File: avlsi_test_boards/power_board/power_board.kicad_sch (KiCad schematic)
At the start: 2 parts, among them J1 PJ-102AH, J2 PJ-102AH

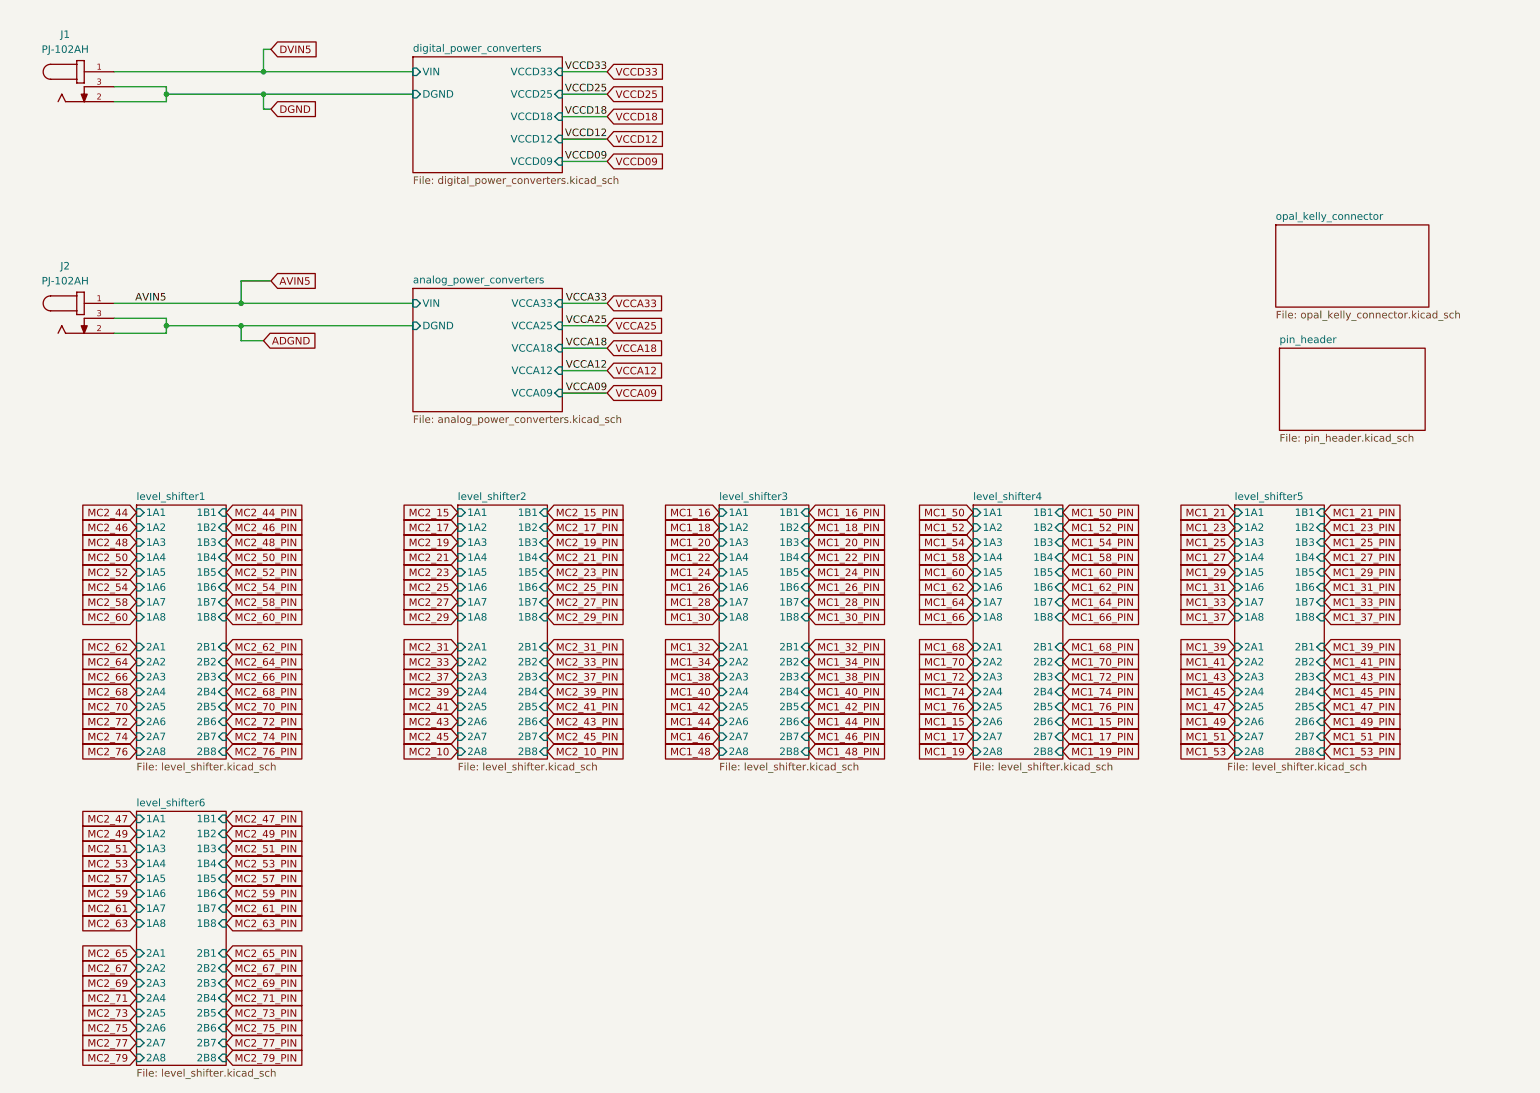
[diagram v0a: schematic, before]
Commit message: Update schematic
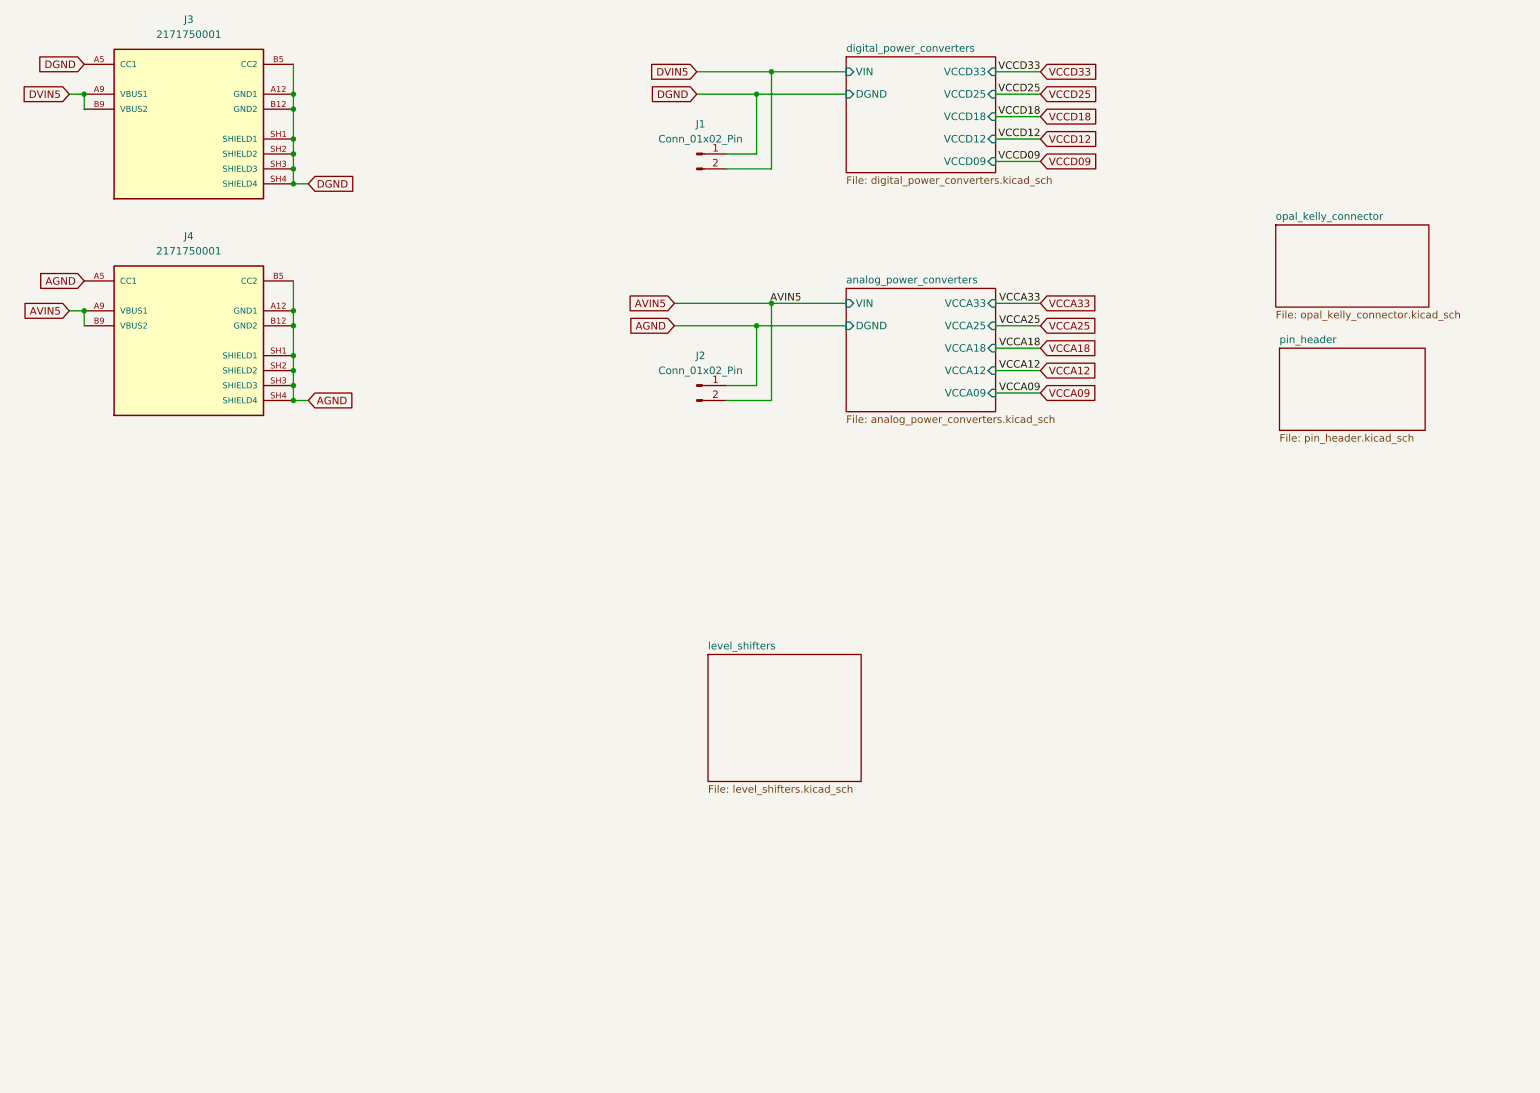
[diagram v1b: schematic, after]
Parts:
- removed J1, J2: PJ-102AH, Connector_BarrelJack:BarrelJack_CUI_PJ-102AH_Horizontal, symbol AVLSI:PJ-102AH
- added J1, J2: Conn_01x02_Pin, Connector_PinHeader_2.54mm:PinHeader_1x02_P2.54mm_Horizontal, symbol Connector:Conn_01x02_Pin
- added J3, J4: 2171750001, avlsi_preferred_parts:MOLEX_2171750001, symbol avlsi_preferred_parts:2171750001
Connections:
- net AVIN5: now also J2.2 (Pin_2), J4.A9 (VBUS1), J4.B9 (VBUS2)
- net DGND: now also J1.1 (Pin_1), J3.A12 (GND1), J3.A5 (CC1), J3.B12 (GND2), J3.B5 (CC2), J3.SH1 (SHIELD1), J3.SH2 (SHIELD2), J3.SH3 (SHIELD3), J3.SH4 (SHIELD4)
- net DVIN5: now also J1.2 (Pin_2), J3.A9 (VBUS1), J3.B9 (VBUS2)
- new net AGND: J2.1 (Pin_1), J4.A12 (GND1), J4.A5 (CC1), J4.B12 (GND2), J4.B5 (CC2), J4.SH1 (SHIELD1), J4.SH2 (SHIELD2), J4.SH3 (SHIELD3), J4.SH4 (SHIELD4)
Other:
- removed sheet level_shifter1
- removed sheet level_shifter2
- removed sheet level_shifter3
- removed sheet level_shifter4
- removed sheet level_shifter5
- removed sheet level_shifter6
- added sheet level_shifters (level_shifters.kicad_sch)
